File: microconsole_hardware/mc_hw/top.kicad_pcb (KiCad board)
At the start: 2 copper layers, 161 x 96 mm, 110 parts, among them J1 USB_C_Receptacle_USB2.0_16P, Q1 Q_PMOS_GSD, SW1 SW_Nidec_CAS-120A1, SW10 TL3301NF160QG, SW11 TL3301NF160QG, SW12 TL3301NF160QG, SW13 TL3301NF160QG, SW14 TL3301NF160QG, SW15 TL3301NF160QG, SW16 Joystick, SW17 Joystick, SW2 TL3301NF160QG, SW3 TL3301NF160QG, SW4 TL3301NF160QG, SW5 TL3301NF160QG, SW6 TL3301NF160QG, SW7 TL3301NF160QG, SW8 TL3301NF160QG, SW9 TL3301NF160QG, U1 MCP73833_MSOP, U2 S2B-PH-K-S, U3 MCP23017-E/SO, U4 ADS7828E/2K5, U5 PCM5102APWR, U6 PAM8302AADCR, U7 PAM8406DR

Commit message: cleanup
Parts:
- C14, C16, C36, C40: value 100nF -> 100nF 50V X7R
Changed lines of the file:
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@@
 	)
 	(footprint "Button_Switch_SMD:Nidec_Copal_CAS-120A"
+		(locked yes)
 		(layer "F.Cu")
 		(at 132 60.5 -90)
@@
 				(font
 					(size 1.27 1.27)
+					(thickness 0.15)
 				)
 			)
@@
 				(font
 					(size 1.27 1.27)
+					(thickness 0.15)
 				)
 			)
@@
 				(font
 					(size 1.27 1.27)
+					(thickness 0.15)
 				)
 			)
@@
 				(font
 					(size 1.27 1.27)
+					(thickness 0.15)
 				)
 			)
@@
 				(font
 					(size 1.27 1.27)
+					(thickness 0.15)
 				)
 				(justify mirror)
@@
 				(font
 					(size 1.27 1.27)
+					(thickness 0.15)
 				)
 				(justify mirror)
@@
 			)
 		)
-		(property "Value" "100nF"
+		(property "Value" "100nF 50V X7R"
 			(at -0.6 -2 90)
 			(layer "B.Fab")
@@
 		)
 		(embedded_fonts no)
-		(model "${KICAD8_3DMODEL_DIR}/Capacitor_SMD.3dshapes/C_0805_2012Metric.wrl"
+		(model "${KICAD10_3DMODEL_DIR}/Capacitor_SMD.3dshapes/C_0805_2012Metric.step"
 			(offset
 				(xyz 0 0 0)
@@
 			)
 		)
-		(property "Value" "100nF"
+		(property "Value" "100nF 50V X7R"
 			(at 0 2 90)
 			(layer "B.Fab")
@@
 		)
 		(embedded_fonts no)
-		(model "${KICAD8_3DMODEL_DIR}/Capacitor_SMD.3dshapes/C_0805_2012Metric.wrl"
+		(model "${KICAD10_3DMODEL_DIR}/Capacitor_SMD.3dshapes/C_0805_2012Metric.step"
 			(offset
 				(xyz 0 0 0)
@@
 			)
 		)
-		(property "Value" "100nF"
+		(property "Value" "100nF 50V X7R"
 			(at 4.1 0.3 0)
 			(layer "B.Fab")
@@
 		)
 		(embedded_fonts no)
-		(model "${KICAD8_3DMODEL_DIR}/Capacitor_SMD.3dshapes/C_0805_2012Metric.wrl"
+		(model "${KICAD10_3DMODEL_DIR}/Capacitor_SMD.3dshapes/C_0805_2012Metric.step"
 			(offset
 				(xyz 0 0 0)
@@
 				(font
 					(size 1.27 1.27)
+					(thickness 0.15)
 				)
 				(justify mirror)
@@
 			)
 		)
-		(property "Value" "100nF"
+		(property "Value" "100nF 50V X7R"
 			(at -3.6 -1.5 90)
 			(layer "B.Fab")
@@
 		)
 		(embedded_fonts no)
-		(model "${KICAD8_3DMODEL_DIR}/Capacitor_SMD.3dshapes/C_0805_2012Metric.wrl"
+		(model "${KICAD10_3DMODEL_DIR}/Capacitor_SMD.3dshapes/C_0805_2012Metric.step"
 			(offset
 				(xyz 0 0 0)
@@
 				(font
 					(size 1.27 1.27)
+					(thickness 0.15)
 				)
 				(justify mirror)
@@
 				(font
 					(size 1.27 1.27)
+					(thickness 0.15)
 				)
 				(justify mirror)
@@
 		)
 		(embedded_fonts no)
-		(model "${KICAD8_3DMODEL_DIR}/Capacitor_SMD.3dshapes/C_0805_2012Metric.wrl"
+		(model "${KICAD10_3DMODEL_DIR}/Capacitor_SMD.3dshapes/C_0805_2012Metric.step"
 			(offset
 				(xyz 0 0 0)
@@
 		)
 		(embedded_fonts no)
-		(model "${KICAD8_3DMODEL_DIR}/Capacitor_SMD.3dshapes/C_0805_2012Metric.wrl"
+		(model "${KICAD10_3DMODEL_DIR}/Capacitor_SMD.3dshapes/C_0805_2012Metric.step"
 			(offset
 				(xyz 0 0 0)
@@
 		)
 		(embedded_fonts no)
-		(model "${KICAD8_3DMODEL_DIR}/Capacitor_SMD.3dshapes/C_0805_2012Metric.wrl"
+		(model "${KICAD10_3DMODEL_DIR}/Capacitor_SMD.3dshapes/C_0805_2012Metric.step"
 			(offset
 				(xyz 0 0 0)
@@
 				(font
 					(size 1.27 1.27)
+					(thickness 0.15)
 				)
 				(justify mirror)
@@
 				(font
 					(size 1.27 1.27)
+					(thickness 0.15)
 				)
 				(justify mirror)
@@
 		)
 		(embedded_fonts no)
-		(model "${KICAD8_3DMODEL_DIR}/Capacitor_SMD.3dshapes/C_0805_2012Metric.wrl"
+		(model "${KICAD10_3DMODEL_DIR}/Capacitor_SMD.3dshapes/C_0805_2012Metric.step"
 			(offset
 				(xyz 0 0 0)
@@
 				(font
 					(size 1.27 1.27)
+					(thickness 0.15)
 				)
 				(justify mirror)
@@
 		)
 		(embedded_fonts no)
-		(model "${KICAD8_3DMODEL_DIR}/Capacitor_SMD.3dshapes/C_0805_2012Metric.wrl"
+		(model "${KICAD10_3DMODEL_DIR}/Capacitor_SMD.3dshapes/C_0805_2012Metric.step"
 			(offset
 				(xyz 0 0 0)
@@
 		)
 		(embedded_fonts no)
-		(model "${KICAD8_3DMODEL_DIR}/Capacitor_SMD.3dshapes/C_0805_2012Metric.wrl"
+		(model "${KICAD10_3DMODEL_DIR}/Capacitor_SMD.3dshapes/C_0805_2012Metric.step"
 			(offset
 				(xyz 0 0 0)
@@
 		)
 		(embedded_fonts no)
-		(model "${KICAD8_3DMODEL_DIR}/Capacitor_SMD.3dshapes/C_0805_2012Metric.wrl"
+		(model "${KICAD10_3DMODEL_DIR}/Capacitor_SMD.3dshapes/C_0805_2012Metric.step"
 			(offset
 				(xyz 0 0 0)
@@
 				(font
 					(size 1.27 1.27)
+					(thickness 0.15)
 				)
 				(justify mirror)
@@
 				(font
 					(size 1.27 1.27)
+					(thickness 0.15)
 				)
 				(justify mirror)
@@
 		)
 		(embedded_fonts no)
-		(model "${KICAD8_3DMODEL_DIR}/Capacitor_SMD.3dshapes/C_0805_2012Metric.wrl"
+		(model "${KICAD10_3DMODEL_DIR}/Capacitor_SMD.3dshapes/C_0805_2012Metric.step"
 			(offset
 				(xyz 0 0 0)
@@
 				(font
 					(size 1.27 1.27)
+					(thickness 0.15)
 				)
 				(justify mirror)
@@
 				(font
 					(size 1.27 1.27)
+					(thickness 0.15)
 				)
 				(justify mirror)
@@
 				(font
 					(size 1.27 1.27)
+					(thickness 0.15)
 				)
 				(justify mirror)
@@
 				(font
 					(size 1.27 1.27)
+					(thickness 0.15)
 				)
 				(justify mirror)
@@
 				(font
 					(size 1.27 1.27)
+					(thickness 0.15)
 				)
 				(justify mirror)
@@
 		)
 		(embedded_fonts no)
-		(model "${KICAD8_3DMODEL_DIR}/Capacitor_SMD.3dshapes/C_0805_2012Metric.wrl"
+		(model "${KICAD10_3DMODEL_DIR}/Capacitor_SMD.3dshapes/C_0805_2012Metric.step"
 			(offset
 				(xyz 0 0 0)

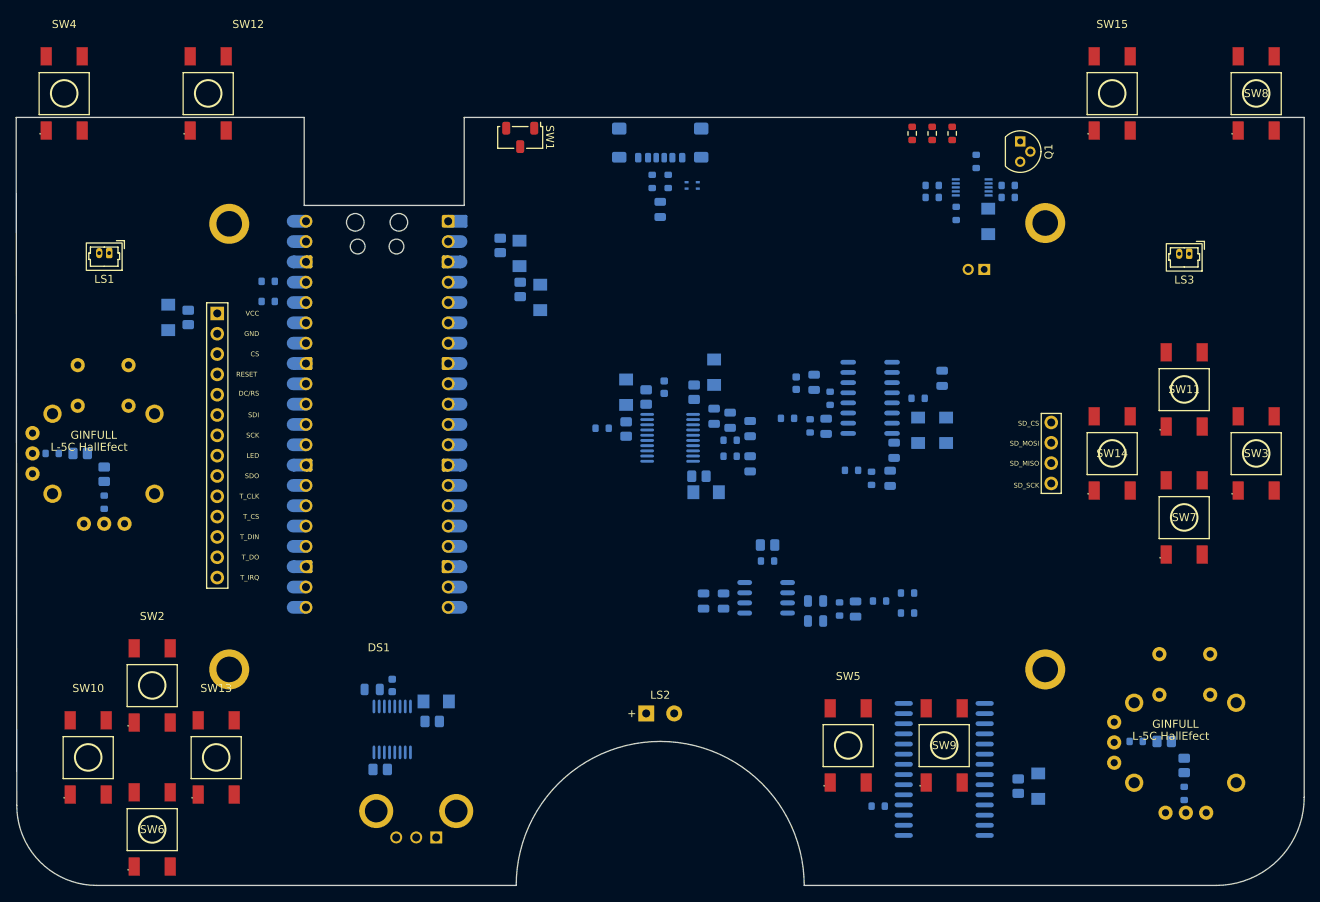
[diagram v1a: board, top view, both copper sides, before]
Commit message: freerouting pass
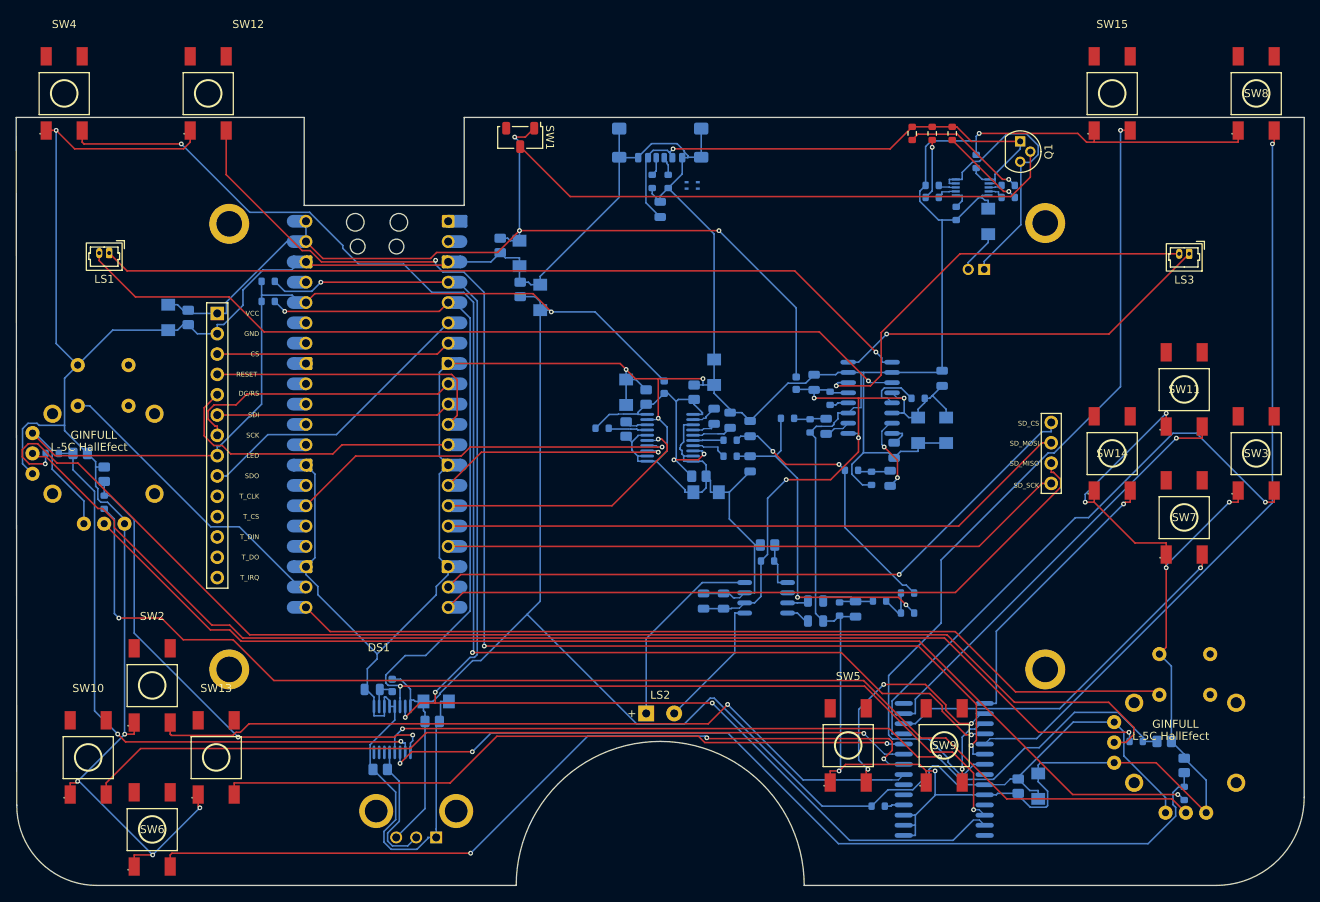
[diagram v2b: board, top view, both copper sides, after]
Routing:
- net GND: track 0.00 -> 914.9 mm, vias 0 -> 15
- net 3v3: track 0.00 -> 315.9 mm, vias 0 -> 1
- net MCP GPB3 / L1: track 0.00 -> 171.5 mm, vias 0 -> 3
- net GPIO3 / MCP|ADC SCL: track 0.00 -> 164.6 mm, vias 0 -> 3
- net IO1 / Left Stick Y: track 0.00 -> 163.1 mm, vias 0 -> 1
- net GPIO2 / MCP|ADC SDA: track 0.00 -> 163.0 mm, vias 0 -> 4
- net MCP GPB5 / L2: track 0.00 -> 161.1 mm, vias 0 -> 3
- net IO0 / Left Stick X: track 0.00 -> 157.9 mm, vias 0 -> 1
- net IO3 / Right Stick Y: track 0.00 -> 153.2 mm, vias 0 -> 1
- net IO2 / Right Stick X: track 0.00 -> 149.3 mm, vias 0 -> 1
- net VSYS_BAT: track 0.00 -> 120.4 mm, vias 0 -> 3
- net FILTERED - IO2 / Right Stick X: track 0.00 -> 113.6 mm, vias 0 -> 2
- net GPIO16 / Left Stick: track 0.00 -> 112.1 mm
- net Net-(LS1--_(black)): track 0.00 -> 106.4 mm, vias 0 -> 1
- net FILTERED - IO3 / Right Stick Y: track 0.00 -> 105.7 mm, vias 0 -> 2
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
